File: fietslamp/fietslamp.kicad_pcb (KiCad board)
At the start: 2 copper layers, 66.5 x 87.4 mm, 21 parts, among them CON14 BED_Th, J1 ADXL, J1 LCD, J12 LED, J2 TH11, J3 ADXL, J4 ESP, J5 LED, J6 ESP, J7 TH11

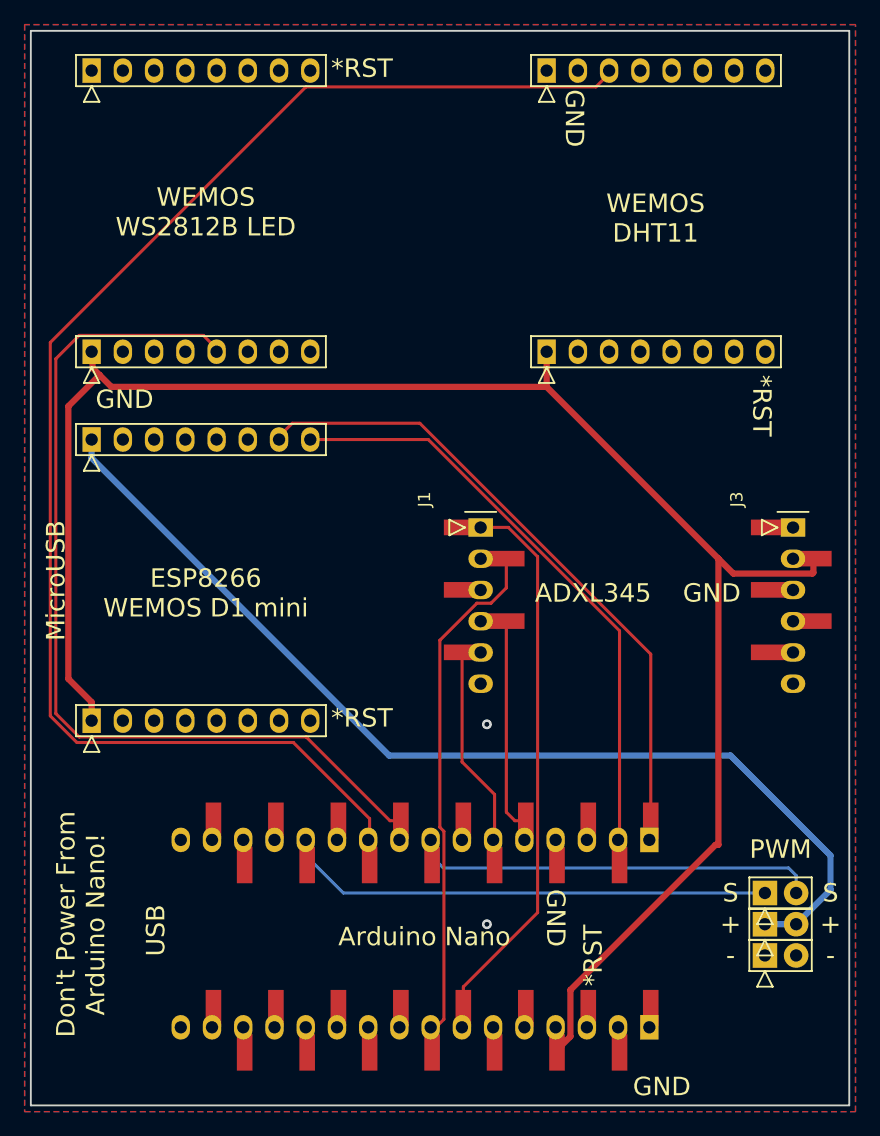
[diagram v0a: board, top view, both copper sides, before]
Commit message: update
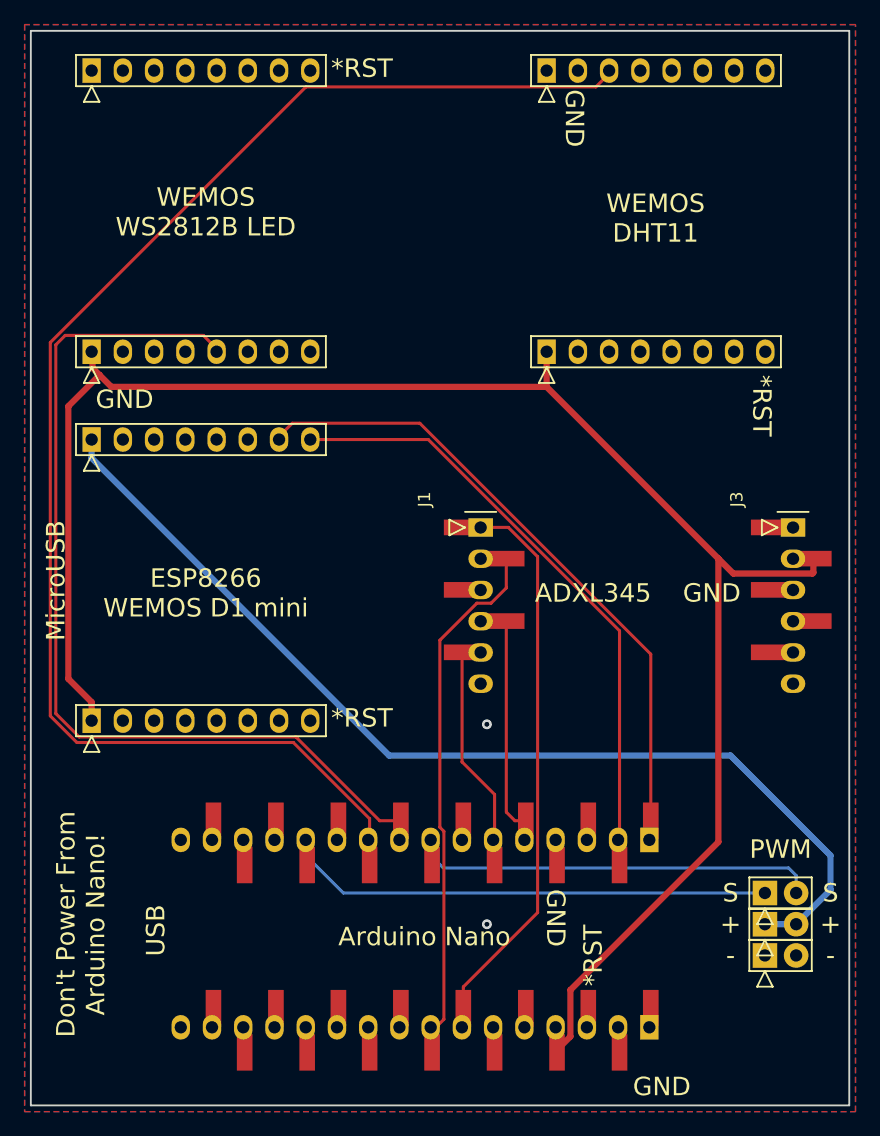
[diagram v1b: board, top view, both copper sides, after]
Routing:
- net Net-(J10-Pad2): track 75.1 -> 75.7 mm
- net (no net): track 193.5 -> 193.0 mm
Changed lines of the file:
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@@
   (segment (start 96.52 107.442) (end 96.52 108.692) (width 0.25) (layer "B.Cu") (net 0))
   (segment (start 139.192 108.712) (end 139.192 111.506) (width 0.508) (layer "B.Cu") (net 0))
-  (segment (start 79.11 74.888) (end 79.11 75.138) (width 0.254) (layer "B.Cu") (net 0))
   (segment (start 107.716 109.728) (end 135.780213 109.728) (width 0.25) (layer "B.Cu") (net 0))
   (segment (start 135.780213 109.728) (end 136.398 110.345787) (width 0.25) (layer "B.Cu") (net 0))
   (segment (start 139.192 111.506) (end 136.398 114.3) (width 0.508) (layer "B.Cu") (net 0))
-  (segment (start 109.22 107.442) (end 109.22 107.692) (width 0.25) (layer "B.Cu") (net 0))
   (segment (start 106.68 107.442) (end 106.68 108.692) (width 0.25) (layer "B.Cu") (net 0))
   (segment (start 106.68 108.692) (end 107.716 109.728) (width 0.25) (layer "B.Cu") (net 0))
@@
   (segment (start 124.576 105.884) (end 124.576 92.343178) (width 0.25) (layer "F.Cu") (net 6))
   (segment (start 105.795812 73.56299) (end 95.42501 73.56299) (width 0.25) (layer "F.Cu") (net 6))
-  (segment (start 94.35 75.138) (end 94.35 74.888) (width 0.25) (layer "F.Cu") (net 6))
   (segment (start 124.576 92.343178) (end 105.795812 73.56299) (width 0.25) (layer "F.Cu") (net 6))
   (segment (start 95.42501 73.56299) (end 94.35 74.638) (width 0.25) (layer "F.Cu") (net 6))
-  (segment (start 78.100008 66.42299) (end 88.19499 66.42299) (width 0.25) (layer "F.Cu") (net 7))
   (segment (start 78.100008 99.07301) (end 76.2 97.173002) (width 0.25) (layer "F.Cu") (net 7))
-  (segment (start 76.2 68.322998) (end 78.100008 66.42299) (width 0.25) (layer "F.Cu") (net 7))
-  (segment (start 104.256 105.884) (end 103.371 105.884) (width 0.25) (layer "F.Cu") (net 7))
-  (segment (start 96.56001 99.07301) (end 78.100008 99.07301) (width 0.25) (layer "F.Cu") (net 7))
+  (segment (start 102.534 105.884) (end 95.72301 99.07301) (width 0.25) (layer "F.Cu") (net 7))
+  (segment (start 76.2 67.183718) (end 76.960728 66.42299) (width 0.25) (layer "F.Cu") (net 7))
+  (segment (start 88.19499 66.42299) (end 89.27 67.498) (width 0.25) (layer "F.Cu") (net 7))
   (segment (start 89.27 67.498) (end 89.27 67.748) (width 0.25) (layer "F.Cu") (net 7))
-  (segment (start 76.2 97.173002) (end 76.2 68.322998) (width 0.25) (layer "F.Cu") (net 7))
-  (segment (start 88.19499 66.42299) (end 89.27 67.498) (width 0.25) (layer "F.Cu") (net 7))
-  (segment (start 103.371 105.884) (end 96.56001 99.07301) (width 0.25) (layer "F.Cu") (net 7))
+  (segment (start 76.960728 66.42299) (end 88.19499 66.42299) (width 0.25) (layer "F.Cu") (net 7))
+  (segment (start 95.72301 99.07301) (end 78.100008 99.07301) (width 0.25) (layer "F.Cu") (net 7))
+  (segment (start 76.2 97.173002) (end 76.2 67.183718) (width 0.25) (layer "F.Cu") (net 7))
+  (segment (start 104.256 105.884) (end 102.534 105.884) (width 0.25) (layer "F.Cu") (net 7))
   (segment (start 79.18501 67.82301) (end 79.11 67.748) (width 0.508) (layer "F.Cu") (net 8))
   (segment (start 77.216 94.346) (end 79.11 96.24) (width 0.508) (layer "F.Cu") (net 8))
   (segment (start 77.216 72.184) (end 77.216 94.346) (width 0.508) (layer "F.Cu") (net 8))
-  (segment (start 118.04401 123.430717) (end 116.956 124.518727) (width 0.508) (layer "F.Cu") (net 8))
-  (segment (start 116.956 124.518727) (end 116.956 124.724) (width 0.508) (layer "F.Cu") (net 8))
-  (segment (start 130.076293 107.843705) (end 130.076293 84.572) (width 0.508) (layer "F.Cu") (net 8))
+  (segment (start 130.076293 84.572) (end 130.076293 107.611505) (width 0.508) (layer "F.Cu") (net 8))
   (segment (start 116.11 70.605707) (end 116.11 67.748) (width 0.508) (layer "F.Cu") (net 8))
-  (segment (start 116.11 67.748) (end 116.11 67.998) (width 0.25) (layer "F.Cu") (net 8))
   (segment (start 137.8 85.715) (end 137.8 84.572) (width 0.508) (layer "F.Cu") (net 8))
   (segment (start 79.756 69.644) (end 79.18501 69.07301) (width 0.508) (layer "F.Cu") (net 8))
+  (segment (start 118.04401 123.430717) (end 116.956 124.518727) (width 0.508) (layer "F.Cu") (net 8))
   (segment (start 130.076293 84.572) (end 116.11 70.605707) (width 0.508) (layer "F.Cu") (net 8))
-  (segment (start 130.076293 107.843705) (end 129.844093 107.843705) (width 0.508) (layer "F.Cu") (net 8))
   (segment (start 79.11 96.24) (end 79.11 97.748) (width 0.508) (layer "F.Cu") (net 8))
-  (segment (start 118.04401 119.643788) (end 118.04401 123.430717) (width 0.508) (layer "F.Cu") (net 8))
   (segment (start 131.290303 85.78601) (end 137.72899 85.78601) (width 0.508) (layer "F.Cu") (net 8))
   (segment (start 79.756 69.644) (end 77.216 72.184) (width 0.508) (layer "F.Cu") (net 8))
-  (segment (start 79.18501 69.07301) (end 79.11 68.998) (width 0.25) (layer "F.Cu") (net 8))
+  (segment (start 116.956 124.518727) (end 116.956 124.724) (width 0.508) (layer "F.Cu") (net 8))
+  (segment (start 118.04401 119.643788) (end 118.04401 123.430717) (width 0.508) (layer "F.Cu") (net 8))
   (segment (start 80.717707 70.605707) (end 79.756 69.644) (width 0.508) (layer "F.Cu") (net 8))
   (segment (start 116.11 70.605707) (end 80.717707 70.605707) (width 0.508) (layer "F.Cu") (net 8))
+  (segment (start 130.076293 107.611505) (end 118.04401 119.643788) (width 0.508) (layer "F.Cu") (net 8))
   (segment (start 130.076293 84.572) (end 131.290303 85.78601) (width 0.508) (layer "F.Cu") (net 8))
   (segment (start 137.72899 85.78601) (end 137.8 85.715) (width 0.508) (layer "F.Cu") (net 8))
   (segment (start 79.18501 69.07301) (end 79.18501 67.82301) (width 0.508) (layer "F.Cu") (net 8))
-  (segment (start 129.844093 107.843705) (end 118.04401 119.643788) (width 0.508) (layer "F.Cu") (net 8))
   (zone (net 1) (net_name "GND") (layer "F.Cu") (hatch edge 0.508)
     (connect_pads (clearance 0.508))

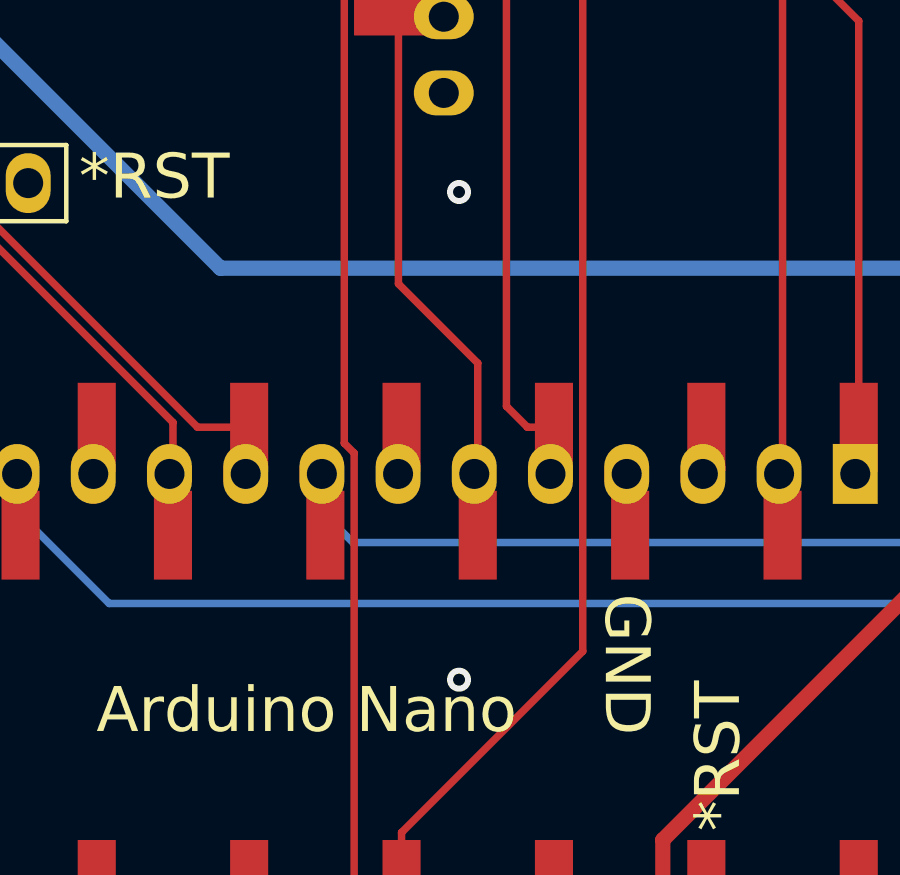
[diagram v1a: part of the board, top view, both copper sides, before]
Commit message: save
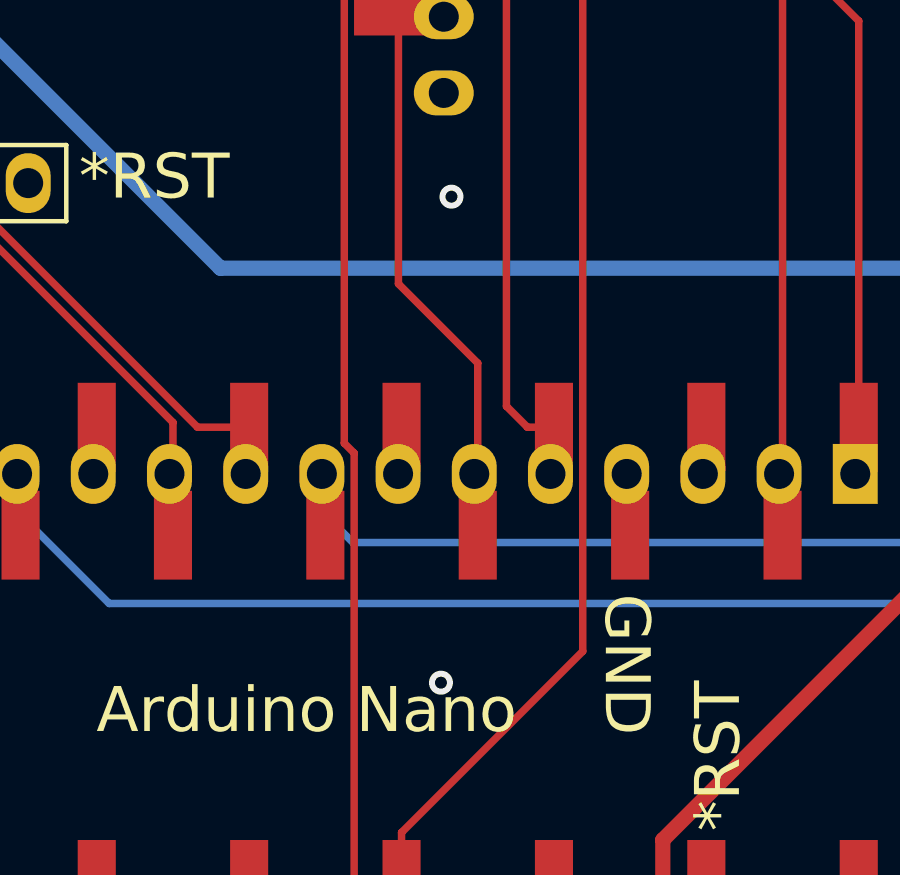
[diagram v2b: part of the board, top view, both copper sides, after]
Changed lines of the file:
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@@
   (segment (start 106.68 108.692) (end 107.716 109.728) (width 0.25) (layer "B.Cu") (net 0))
   (segment (start 136.398 110.345787) (end 136.398 111.76) (width 0.25) (layer "B.Cu") (net 0))
-  (via (at 111.252 114.3) (size 0.8) (drill 0.4) (layers "F.Cu" "B.Cu") (net 1))
-  (via (at 111.252 98.044) (size 0.8) (drill 0.4) (layers "F.Cu" "B.Cu") (net 1))
+  (via (at 110.65 114.4) (size 0.8) (drill 0.4) (layers "F.Cu" "B.Cu") (net 1))
+  (via (at 111 98.2) (size 0.8) (drill 0.4) (layers "F.Cu" "B.Cu") (net 1))
   (segment (start 115.376001 84.415999) (end 112.992002 82.032) (width 0.25) (layer "F.Cu") (net 2))
   (segment (start 109.336 119.394) (end 115.376001 113.353999) (width 0.25) (layer "F.Cu") (net 2))
